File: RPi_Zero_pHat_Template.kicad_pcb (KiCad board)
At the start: 2 copper layers, 65 x 30.5 mm, 6 parts, among them J1 RPi_GPIO, J2 RPi_GPIO

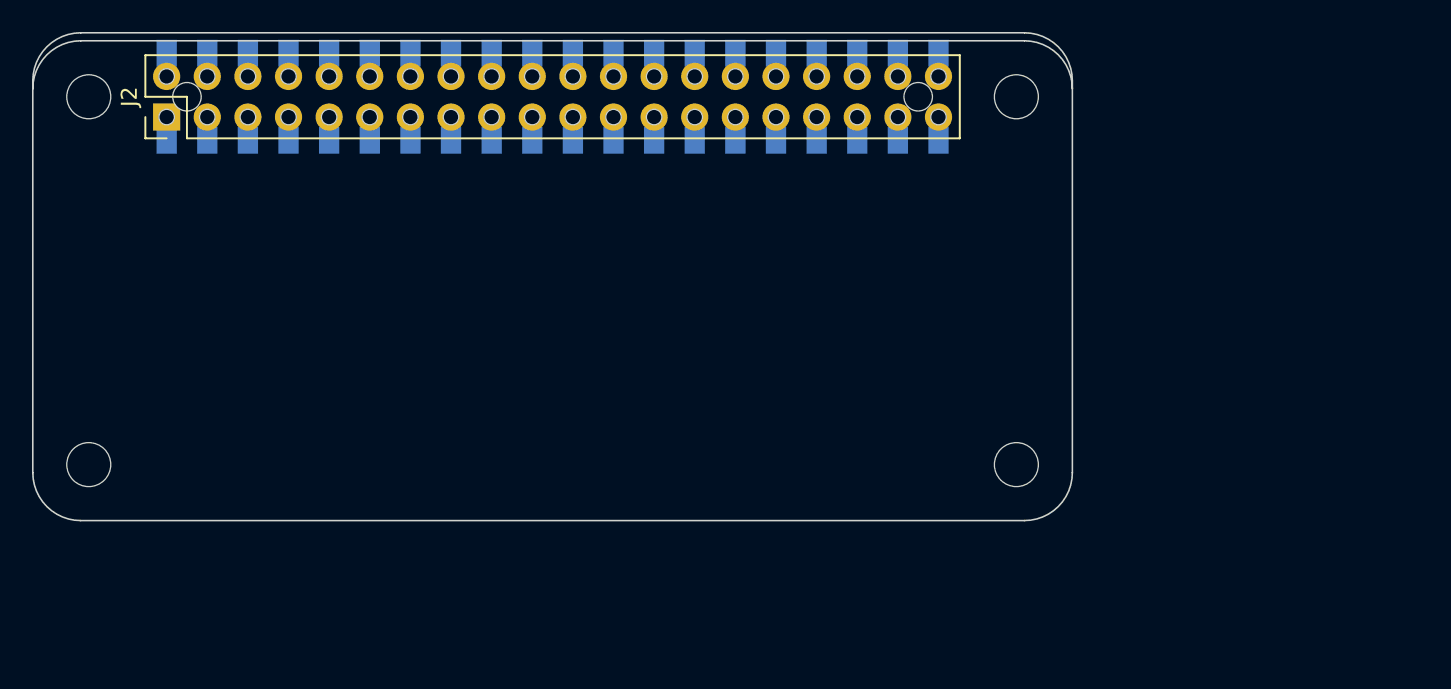
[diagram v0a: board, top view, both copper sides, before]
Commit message: PCB sent out for manufacture.
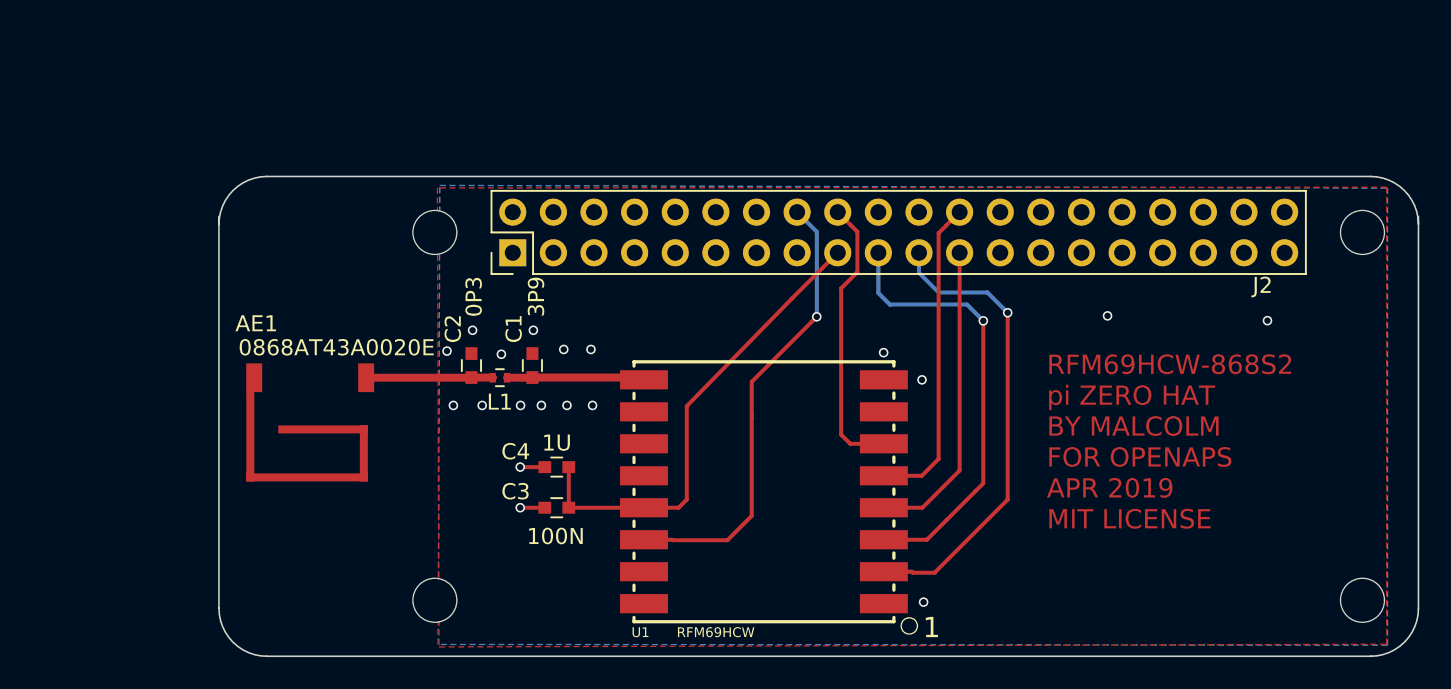
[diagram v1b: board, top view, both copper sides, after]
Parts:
- removed J1: RPi_GPIO, Connector_Samtec_HLE_SMD-ML:Samtec_HLE-120-02-xxx-DV-BE-A_2x20_RPi_Bottom
- added AE1: 0868AT43A0020E, footprints:0868AT43A0020E, F.Cu at (29.8, 45.6)
- added C1: 3P9, Capacitors_SMD:C_0603, F.Cu at (43.7, 44.8)
- added C2: 0P3, Capacitors_SMD:C_0603, F.Cu at (39.9, 44.8)
- added C3: 100N, Capacitors_SMD:C_0603, F.Cu at (45.3, 53.7)
- added C4: 1U, Capacitors_SMD:C_0603, F.Cu at (45.3, 51.2)
- added L1: 18N, Resistors_SMD:R_0402, F.Cu at (41.7, 45.6)
- added REF**: muwave_stub, muwave_stub, F.Cu at (33.2, 48.8)
- added REF** (x2): muwave_stub, muwave_stub, F.Cu at (33.2, 51.8)
- added REF**: muwave_stub, muwave_stub, F.Cu at (26.1, 51.8)
- added U1: RFM69HCW, RF:RFM69HCW-XXXS2, F.Cu at (58.2, 52.7)
- moved J2 23.2 mm to (42.5, 37.8)
- moved ? 23.2 mm to (37.6, 59.5)
- moved ? 23.2 mm to (95.6, 36.5)
- moved ? 23.2 mm to (95.6, 59.5)
- moved ? 23.2 mm to (37.6, 36.5)
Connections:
- J2 pad 14: Net-(J2-Pad14) -> GND
- J2 pad 17: Net-(J2-Pad17) -> +3V3
- J2 pad 25: Net-(J2-Pad25) -> GND
- J2 pad 39: Net-(J2-Pad39) -> GND
- J2 pad 6: Net-(J2-Pad6) -> GND
- J2 pad 9: Net-(J2-Pad9) -> GND
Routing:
- net +3V3: track 0.00 -> 29.4 mm
- net Net-(J2-Pad21): track 0.00 -> 29.2 mm, vias 0 -> 1
- net Net-(J2-Pad16): track 0.00 -> 28.6 mm, vias 0 -> 1
- net Net-(J2-Pad19): track 0.00 -> 27.6 mm, vias 0 -> 1
- net Net-(J2-Pad24): track 0.00 -> 19.8 mm
- net Net-(J2-Pad23): track 0.00 -> 19.3 mm
- net Net-(J2-Pad18): track 0.00 -> 17.7 mm
- net Net-(C1-Pad1): track 0.00 -> 8.63 mm
- net Net-(AE1-Pad2): track 0.00 -> 7.92 mm
- net GND: track 0.00 -> 3.07 mm, vias 0 -> 19
- added copper zone on B.Cu, net GND
- added copper zone on F.Cu, net GND
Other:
- board size 65 x 30.5 mm -> 75 x 30 mm
- net class RF added: clearance 0.2, trace_width 0.5, via_dia 0.6, via_drill 0.4
- board text added: "RFM69HCW-868S2 pi ZERO HAT BY MALCOLM FOR OPENAPS APR 2019 MIT LICENSE"
